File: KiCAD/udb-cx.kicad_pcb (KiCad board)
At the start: 4 copper layers, 18 x 16.5 mm, 15 parts, among them J1 SM04B-SRSS-TB(LF)(SN), J2 USB_C_Receptacle, U1 TPD4E05U06DQAR

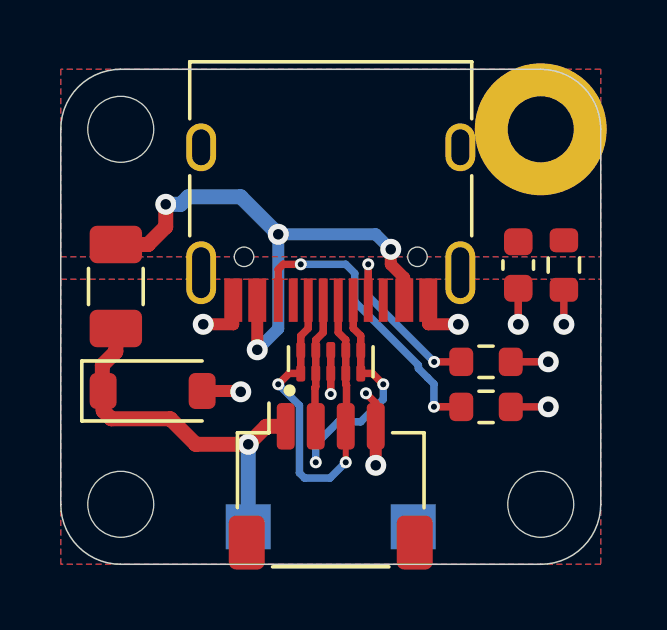
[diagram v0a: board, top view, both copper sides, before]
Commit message: .
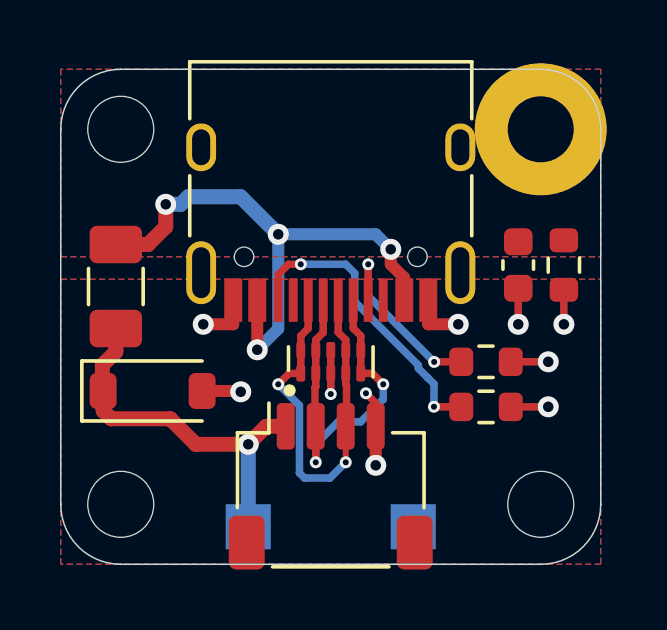
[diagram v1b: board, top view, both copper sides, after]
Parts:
- renumbered TP1 to TP-Gnd1, TP to TP-Vcc1
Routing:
- net D-: track 11.7 -> 12.9 mm
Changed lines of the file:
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@@
 		(descr "SMD rectangular pad as test Point, square 1.5mm side length")
 		(tags "test point SMD pad rectangle square")
-		(property "Reference" "TP1"
+		(property "Reference" "TP-Gnd1"
 			(at 0 1.648 0)
 			(layer "B.SilkS")
@@
 		(descr "SMD rectangular pad as test Point, square 1.5mm side length")
 		(tags "test point SMD pad rectangle square")
-		(property "Reference" "TP"
+		(property "Reference" "TP-Vcc1"
 			(at 0 1.648 0)
 			(layer "B.SilkS")
@@
 	)
 	(segment
+		(start 101.25 44.840721)
+		(end 101.590721 44.5)
+		(width 0.25)
+		(layer "F.Cu")
+		(net 3)
+	)
+	(segment
+		(start 101.25 45.695)
+		(end 101.25 44.840721)
+		(width 0.25)
+		(layer "F.Cu")
+		(net 3)
+	)
+	(segment
 		(start 107.346101 49.247793)
 		(end 107.351528 49.25322)
@@
 	)
 	(segment
-		(start 101.418 44.5)
-		(end 102 44.5)
-		(width 0.25)
-		(layer "F.Cu")
-		(net 3)
-	)
-	(segment
-		(start 101.25 45.695)
-		(end 101.25 44.668)
-		(width 0.25)
-		(layer "F.Cu")
-		(net 3)
-	)
-	(segment
 		(start 106.43974 49.247793)
 		(end 107.346101 49.247793)
@@
 	)
 	(segment
-		(start 101.25 44.668)
-		(end 101.418 44.5)
+		(start 101.590721 44.5)
+		(end 102 44.5)
 		(width 0.25)
 		(layer "F.Cu")
@@
 		(end 102.5 49.9)
 		(width 0.25)
+		(layer "F.Cu")
+		(net 10)
+	)
+	(segment
+		(start 102.5 51.1)
+		(end 102.5 49.9)
+		(width 0.25)
